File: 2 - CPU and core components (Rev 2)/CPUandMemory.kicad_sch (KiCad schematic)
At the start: 9 parts

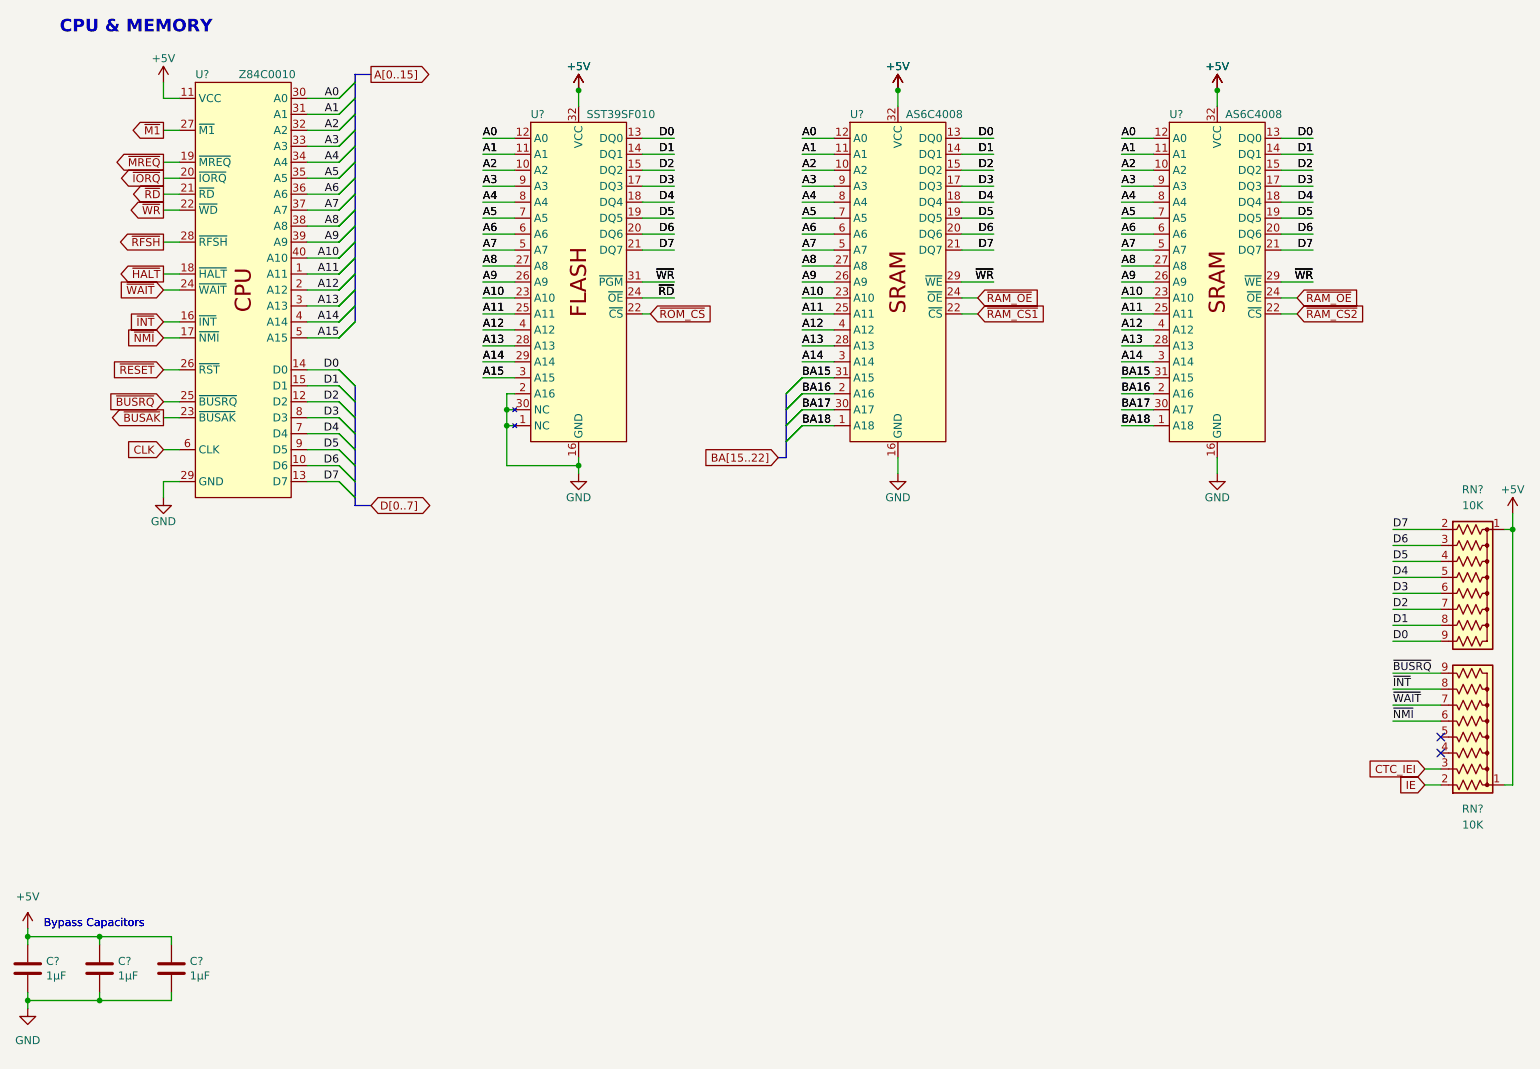
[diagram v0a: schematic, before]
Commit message: Finished component placement, currently routing.
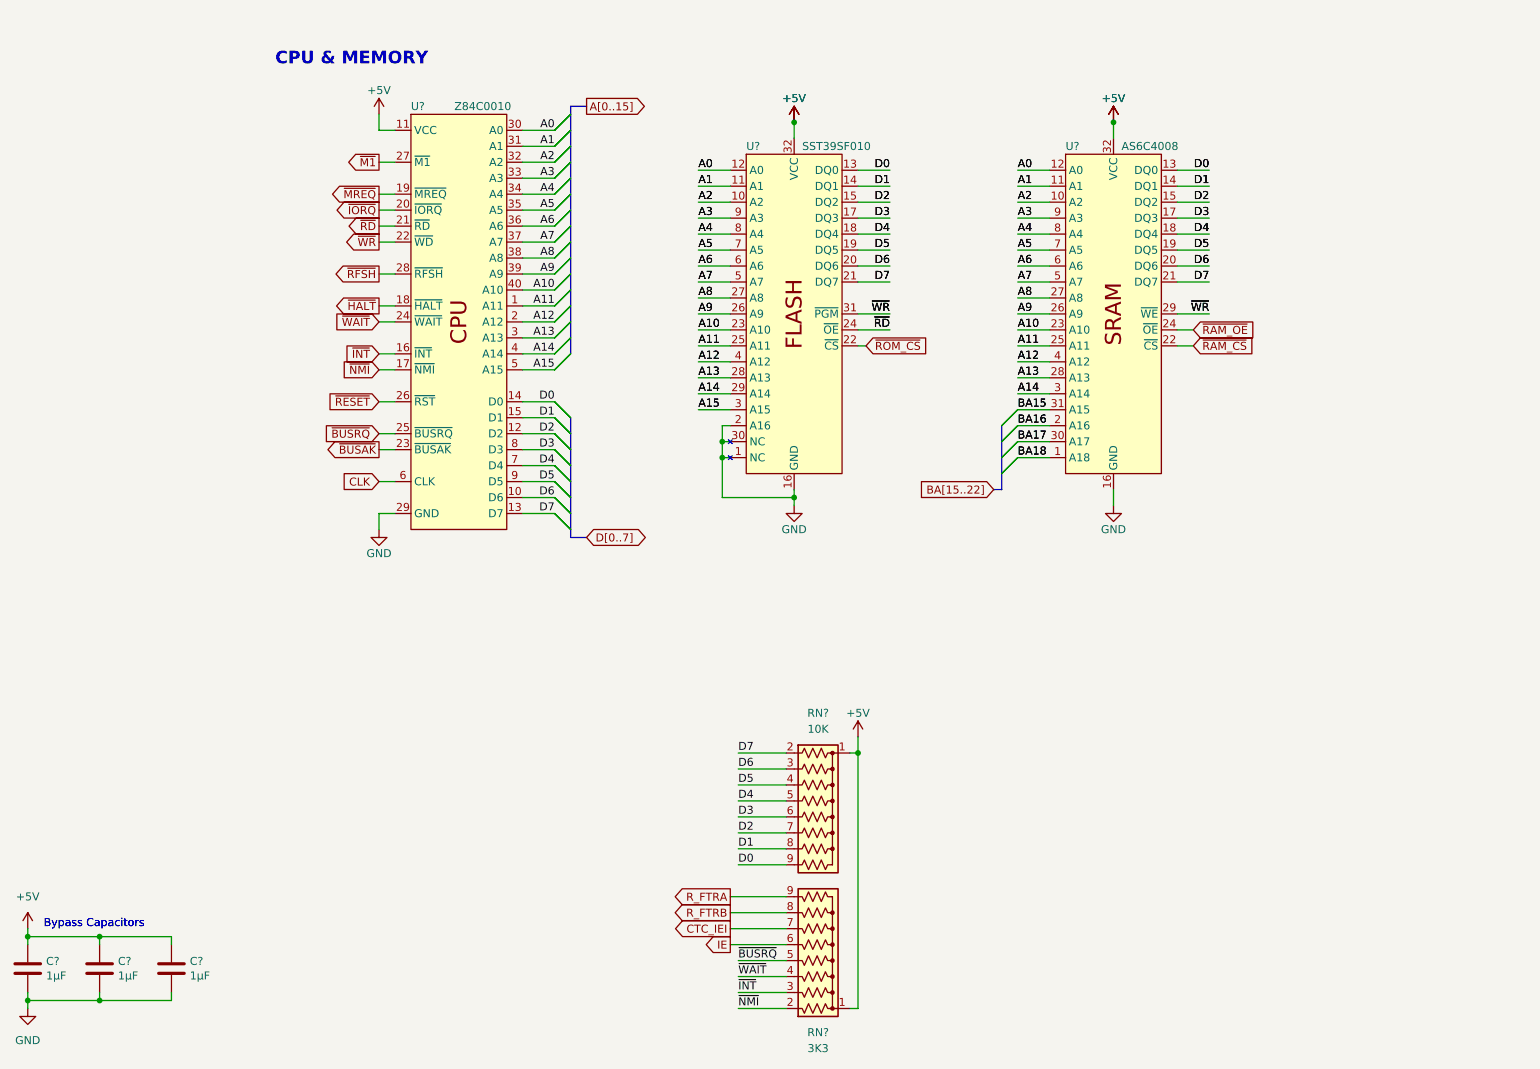
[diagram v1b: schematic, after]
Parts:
- removed U?: AS6C4008, Package_DIP:DIP-32_W15.24mm_Socket, symbol 0_Library:AS6C4008
- RN?: value 10K -> 3K3
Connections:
- net CTC_IEI: now also RN?.7 (R6); no longer RN?.3 (R2)
- net IE: now also RN?.6 (R5); no longer RN?.2 (R1)
- net ~{BUSRQ}: now also RN?.5 (R4); no longer RN?.9 (R8)
- net ~{INT}: now also RN?.3 (R2); no longer RN?.8 (R7)
- net ~{NMI}: now also RN?.2 (R1); no longer RN?.6 (R5)
- net ~{WAIT}: now also RN?.4 (R3); no longer RN?.7 (R6)
- net ~{RAM_CS1} renamed ~{RAM_CS}
- new net R_FTRA: RN?.9 (R8)
- new net R_FTRB: RN?.8 (R7)
- no-connect marks 2 -> 0
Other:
- moved on the sheet: RN?, U?
